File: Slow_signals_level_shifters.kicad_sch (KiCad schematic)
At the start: 34 parts, among them IC3 TCA9406DCUR, IC4 TCA9406DCUR, IC5 TCA9406DCUR, IC7 SN74AVC1T45DCKT, U3 SN74AVCH16T245GR

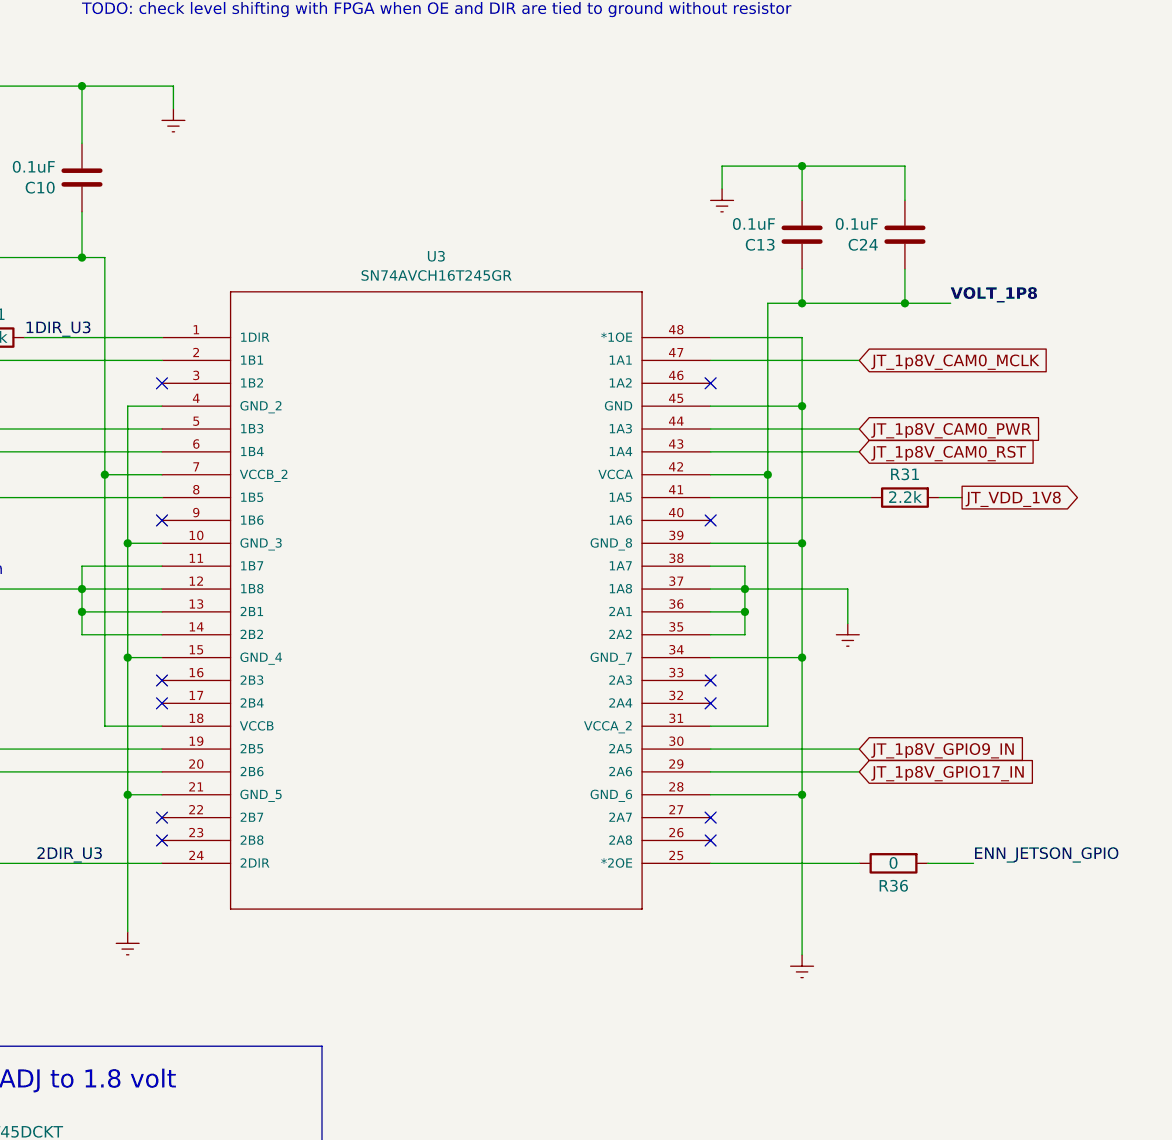
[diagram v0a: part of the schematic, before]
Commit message: All DRC, ERC and BOM are good
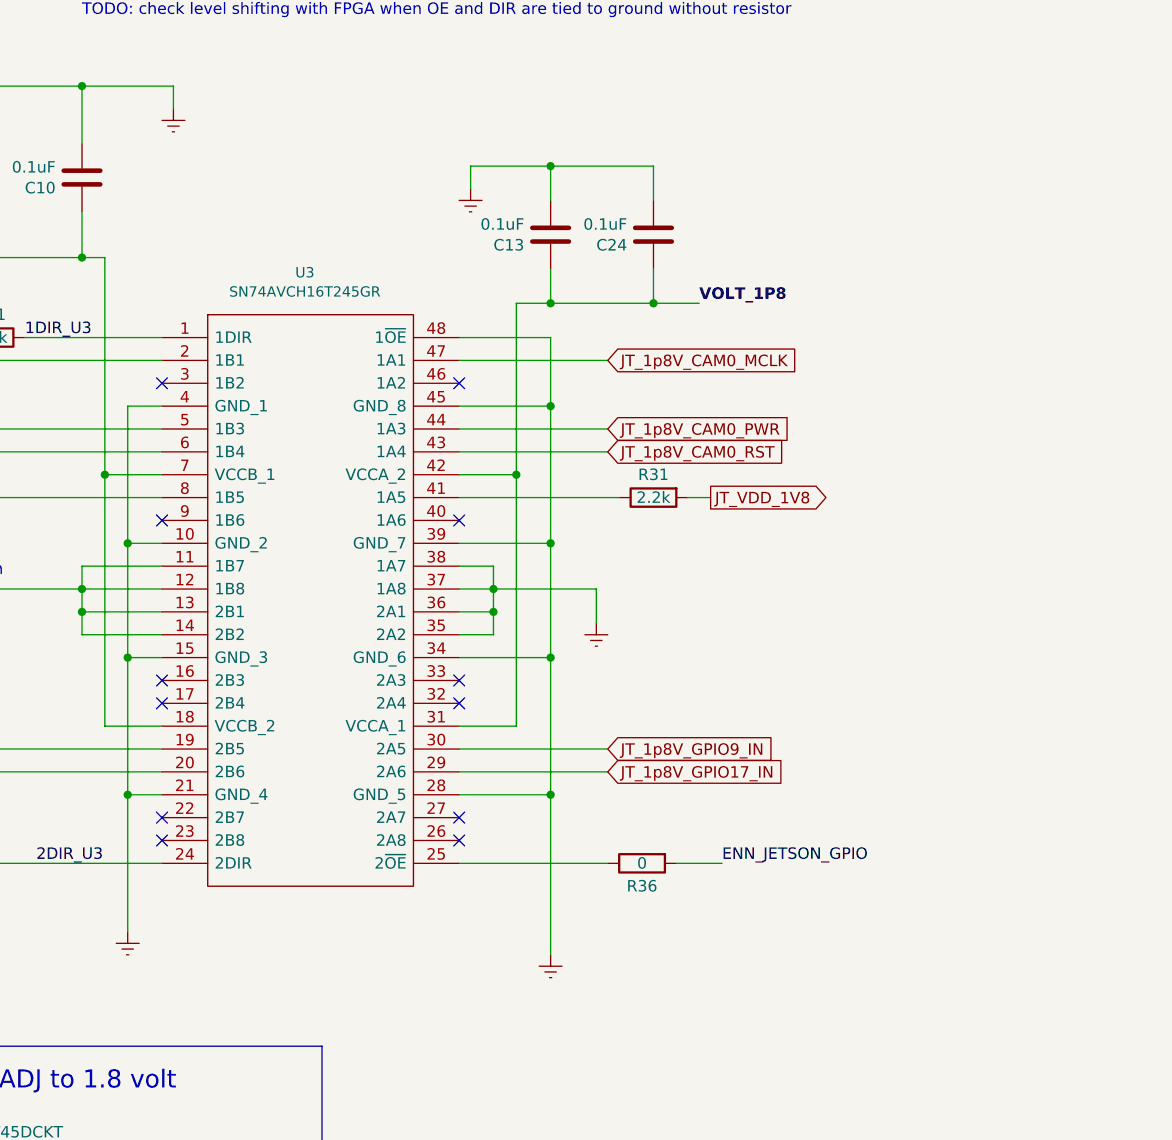
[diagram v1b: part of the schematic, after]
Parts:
- U3: footprint FMC_MIPI_v2_sym:SOP50P810X120-48N -> SOP50P810X120-48N; symbol FMC_MIPI_v2:SN74AVCH16T245_DGV_48 -> FMC_MIPI_v2:SN74AVCH16T245GR; Height (none) -> 1.2; Manufacturer_Name (none) -> Texas Instruments; Manufacturer_Part_Number (none) -> SN74AVCH16T245GR; Mouser Part Number (none) -> 595-SN74AVCH16T245GR; Mouser Price/Stock (none) -> https://www.mouser.co.uk/ProductDetail/Texas-Instruments/SN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
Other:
- moved on the sheet: C13, C24, R31, R36
